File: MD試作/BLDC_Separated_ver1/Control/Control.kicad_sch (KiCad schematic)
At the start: 20 parts, among them J1 Conn_01x14_Pin, J2 Conn_02x13_Odd_Even, SW1 SW_SPST, U1 STM32G473CET6, Y1 16MHz

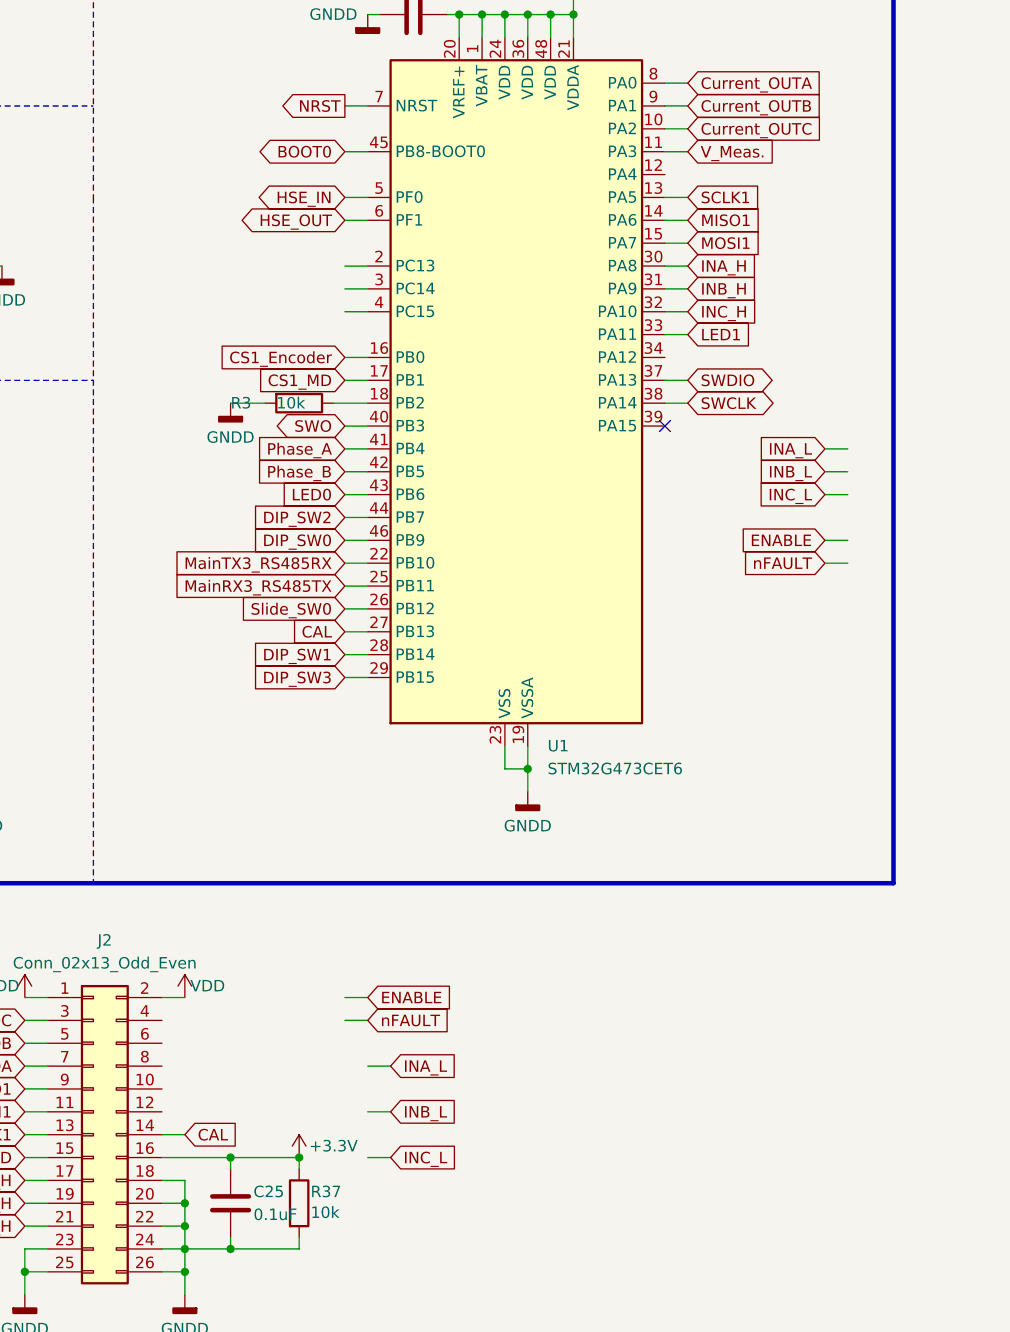
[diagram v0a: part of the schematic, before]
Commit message: かんせい
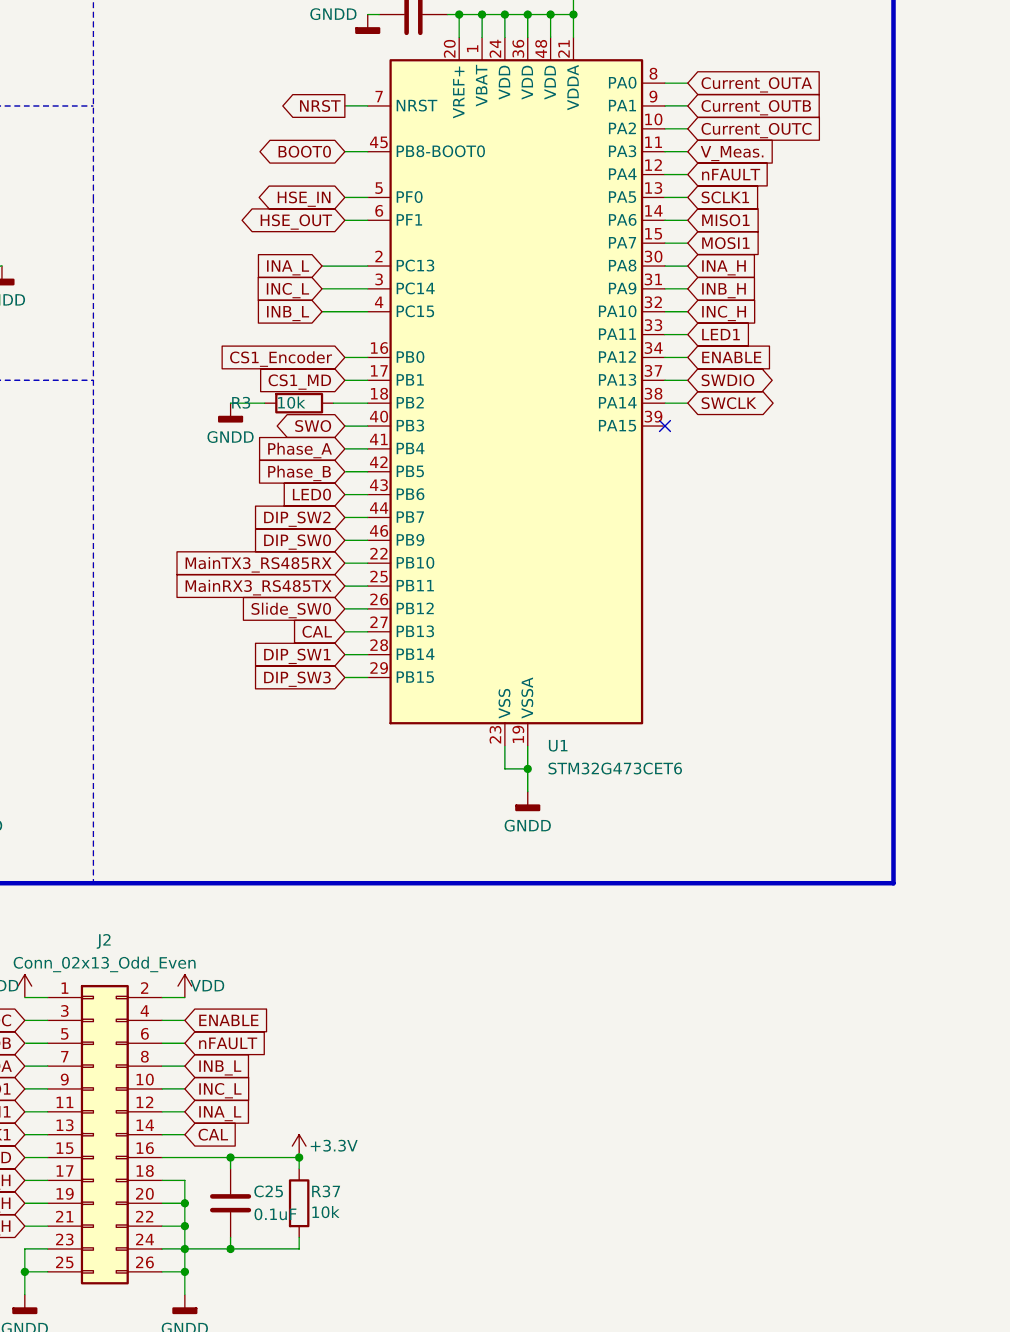
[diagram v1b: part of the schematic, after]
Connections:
- net ENABLE: now also J2.4 (Pin_4), U1.34 (PA12)
- net INA_L: now also J2.12 (Pin_12), U1.2 (PC13)
- net INB_L: now also J2.8 (Pin_8), U1.4 (PC15)
- net INC_L: now also J2.10 (Pin_10), U1.3 (PC14)
- net nFAULT: now also J2.6 (Pin_6), U1.12 (PA4)
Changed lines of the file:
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@@
   (no_connect (at 101.6 119.38))
   (no_connect (at 101.6 116.84))
-  (wire (pts (xy 162.56 175.26) (xy 160.02 175.26))
+  (wire (pts (xy 139.7 180.34) (xy 137.16 180.34))
     (stroke (width 0) (type default))
   )
@@
     (stroke (width 0) (type default))
   )
-  (wire (pts (xy 162.56 185.42) (xy 160.02 185.42))
+  (wire (pts (xy 139.7 177.8) (xy 137.16 177.8))
     (stroke (width 0) (type default))
   )
@@
     (stroke (width 0) (type default))
   )
-  (wire (pts (xy 157.48 88.9) (xy 160.02 88.9))
+  (wire (pts (xy 154.94 88.9) (xy 160.02 88.9))
     (stroke (width 0) (type default))
   )
@@
     (stroke (width 0) (type default))
   )
-  (wire (pts (xy 213.36 109.22) (xy 210.82 109.22))
-    (stroke (width 0) (type default))
-  )
   (wire (pts (xy 124.46 195.58) (xy 121.92 195.58))
     (stroke (width 0) (type default))
@@
     (stroke (width 0) (type default))
   )
-  (wire (pts (xy 157.48 167.64) (xy 160.02 167.64))
-    (stroke (width 0) (type default))
-  )
-  (wire (pts (xy 162.56 180.34) (xy 160.02 180.34))
+  (wire (pts (xy 137.16 170.18) (xy 139.7 170.18))
+    (stroke (width 0) (type default))
+  )
+  (wire (pts (xy 139.7 175.26) (xy 137.16 175.26))
     (stroke (width 0) (type default))
   )
@@
     (stroke (width 0) (type default))
   )
-  (wire (pts (xy 160.02 170.18) (xy 157.48 170.18))
+  (wire (pts (xy 139.7 172.72) (xy 137.16 172.72))
     (stroke (width 0) (type default))
   )
@@
     (stroke (width 0) (type default))
   )
-  (wire (pts (xy 210.82 119.38) (xy 213.36 119.38))
+  (wire (pts (xy 195.58 76.2) (xy 193.04 76.2))
     (stroke (width 0) (type default))
   )
@@
     (stroke (width 0) (type default))
   )
-  (wire (pts (xy 213.36 106.68) (xy 210.82 106.68))
-    (stroke (width 0) (type default))
-  )
   (wire (pts (xy 121.92 177.8) (xy 124.46 177.8))
     (stroke (width 0) (type default))
   )
-  (wire (pts (xy 213.36 116.84) (xy 210.82 116.84))
+  (wire (pts (xy 193.04 96.52) (xy 195.58 96.52))
     (stroke (width 0) (type default))
   )
@@
     (stroke (width 0) (type default))
   )
-  (wire (pts (xy 157.48 86.36) (xy 160.02 86.36))
+  (wire (pts (xy 154.94 86.36) (xy 160.02 86.36))
     (stroke (width 0) (type default))
   )
@@
   )
   (wire (pts (xy 35.56 119.38) (xy 35.56 121.92))
-    (stroke (width 0) (type default))
-  )
-  (wire (pts (xy 213.36 111.76) (xy 210.82 111.76))
     (stroke (width 0) (type default))
   )
@@
     (stroke (width 0) (type default))
   )
-  (wire (pts (xy 157.48 91.44) (xy 160.02 91.44))
+  (wire (pts (xy 154.94 91.44) (xy 160.02 91.44))
     (stroke (width 0) (type default))
   )
@@
     )
   )
-  (global_label "nFAULT" (shape input) (at 160.02 170.18 0) (fields_autoplaced)
-    (effects (font (size 1.27 1.27)) (justify left))
-    (property "Intersheetrefs" "${INTERSHEET_REFS}" (at 169.6576 170.18 0)
+  (global_label "nFAULT" (shape input) (at 139.7 172.72 0) (fields_autoplaced)
+    (effects (font (size 1.27 1.27)) (justify left))
+    (property "Intersheetrefs" "${INTERSHEET_REFS}" (at 149.3376 172.72 0)
       (effects (font (size 1.27 1.27)) (justify left) hide)
     )
@@
     )
   )
-  (global_label "INC_L" (shape input) (at 210.82 111.76 180) (fields_autoplaced)
-    (effects (font (size 1.27 1.27)) (justify right))
-    (property "Intersheetrefs" "${INTERSHEET_REFS}" (at 202.6338 111.76 0)
+  (global_label "INC_L" (shape input) (at 154.94 88.9 180) (fields_autoplaced)
+    (effects (font (size 1.27 1.27)) (justify right))
+    (property "Intersheetrefs" "${INTERSHEET_REFS}" (at 146.7538 88.9 0)
       (effects (font (size 1.27 1.27)) (justify right) hide)
     )
@@
     )
   )
-  (global_label "INB_L" (shape input) (at 210.82 109.22 180) (fields_autoplaced)
-    (effects (font (size 1.27 1.27)) (justify right))
-    (property "Intersheetrefs" "${INTERSHEET_REFS}" (at 202.6338 109.22 0)
+  (global_label "INB_L" (shape input) (at 154.94 91.44 180) (fields_autoplaced)
+    (effects (font (size 1.27 1.27)) (justify right))
+    (property "Intersheetrefs" "${INTERSHEET_REFS}" (at 146.7538 91.44 0)
       (effects (font (size 1.27 1.27)) (justify right) hide)
     )
@@
     )
   )
-  (global_label "INC_L" (shape input) (at 162.56 185.42 0) (fields_autoplaced)
-    (effects (font (size 1.27 1.27)) (justify left))
-    (property "Intersheetrefs" "${INTERSHEET_REFS}" (at 170.7462 185.42 0)
+  (global_label "INC_L" (shape input) (at 139.7 177.8 0) (fields_autoplaced)
+    (effects (font (size 1.27 1.27)) (justify left))
+    (property "Intersheetrefs" "${INTERSHEET_REFS}" (at 147.8862 177.8 0)
       (effects (font (size 1.27 1.27)) (justify left) hide)
     )
@@
     )
   )
-  (global_label "ENABLE" (shape input) (at 160.02 167.64 0) (fields_autoplaced)
-    (effects (font (size 1.27 1.27)) (justify left))
-    (property "Intersheetrefs" "${INTERSHEET_REFS}" (at 170.0204 167.64 0)
+  (global_label "ENABLE" (shape input) (at 139.7 170.18 0) (fields_autoplaced)
+    (effects (font (size 1.27 1.27)) (justify left))
+    (property "Intersheetrefs" "${INTERSHEET_REFS}" (at 149.7004 170.18 0)
       (effects (font (size 1.27 1.27)) (justify left) hide)
     )
@@
     )
   )
-  (global_label "INB_L" (shape input) (at 162.56 180.34 0) (fields_autoplaced)
-    (effects (font (size 1.27 1.27)) (justify left))
-    (property "Intersheetrefs" "${INTERSHEET_REFS}" (at 170.7462 180.34 0)
+  (global_label "INB_L" (shape input) (at 139.7 175.26 0) (fields_autoplaced)
+    (effects (font (size 1.27 1.27)) (justify left))
+    (property "Intersheetrefs" "${INTERSHEET_REFS}" (at 147.8862 175.26 0)
       (effects (font (size 1.27 1.27)) (justify left) hide)
     )
@@
     )
   )
-  (global_label "ENABLE" (shape input) (at 210.82 116.84 180) (fields_autoplaced)
-    (effects (font (size 1.27 1.27)) (justify right))
-    (property "Intersheetrefs" "${INTERSHEET_REFS}" (at 200.8196 116.84 0)
-      (effects (font (size 1.27 1.27)) (justify right) hide)
+  (global_label "ENABLE" (shape input) (at 195.58 96.52 0) (fields_autoplaced)
+    (effects (font (size 1.27 1.27)) (justify left))
+    (property "Intersheetrefs" "${INTERSHEET_REFS}" (at 205.5804 96.52 0)
+      (effects (font (size 1.27 1.27)) (justify left) hide)
     )
   )
@@
     )
   )
-  (global_label "INA_L" (shape input) (at 162.56 175.26 0) (fields_autoplaced)
-    (effects (font (size 1.27 1.27)) (justify left))
-    (property "Intersheetrefs" "${INTERSHEET_REFS}" (at 170.5648 175.26 0)
+  (global_label "INA_L" (shape input) (at 139.7 180.34 0) (fields_autoplaced)
+    (effects (font (size 1.27 1.27)) (justify left))
+    (property "Intersheetrefs" "${INTERSHEET_REFS}" (at 147.7048 180.34 0)
       (effects (font (size 1.27 1.27)) (justify left) hide)
     )
@@
     )
   )
-  (global_label "nFAULT" (shape input) (at 210.82 119.38 180) (fields_autoplaced)
-    (effects (font (size 1.27 1.27)) (justify right))
-    (property "Intersheetrefs" "${INTERSHEET_REFS}" (at 201.1824 119.38 0)
-      (effects (font (size 1.27 1.27)) (justify right) hide)
+  (global_label "nFAULT" (shape input) (at 195.58 76.2 0) (fields_autoplaced)
+    (effects (font (size 1.27 1.27)) (justify left))
+    (property "Intersheetrefs" "${INTERSHEET_REFS}" (at 205.2176 76.2 0)
+      (effects (font (size 1.27 1.27)) (justify left) hide)
     )
   )
@@
     )
   )
-  (global_label "INA_L" (shape input) (at 210.82 106.68 180) (fields_autoplaced)
-    (effects (font (size 1.27 1.27)) (justify right))
-    (property "Intersheetrefs" "${INTERSHEET_REFS}" (at 202.8152 106.68 0)
-      (effects (font (size 1.27 1.27)) (justify right) hide)
-    )
+  (global_label "INA_L" (shape input) (at 154.94 86.36 180) (fields_autoplaced)
+    (effects (font (size 1.27 1.27)) (justify right))
+    (property "Intersheetrefs" "${INTERSHEET_REFS}" (at 146.9352 86.36 0)
+      (effects (font (size 1.27 1.27)) (justify right) hide)
+    )
